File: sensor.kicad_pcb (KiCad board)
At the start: 2 copper layers, 42.2 x 40.8 mm, 14 parts, among them J1 Conn_01x06_Female, U2 TLV70019_SOT23-5, U3 TXB0106PWR, U4 PMW3360DM-T2QU

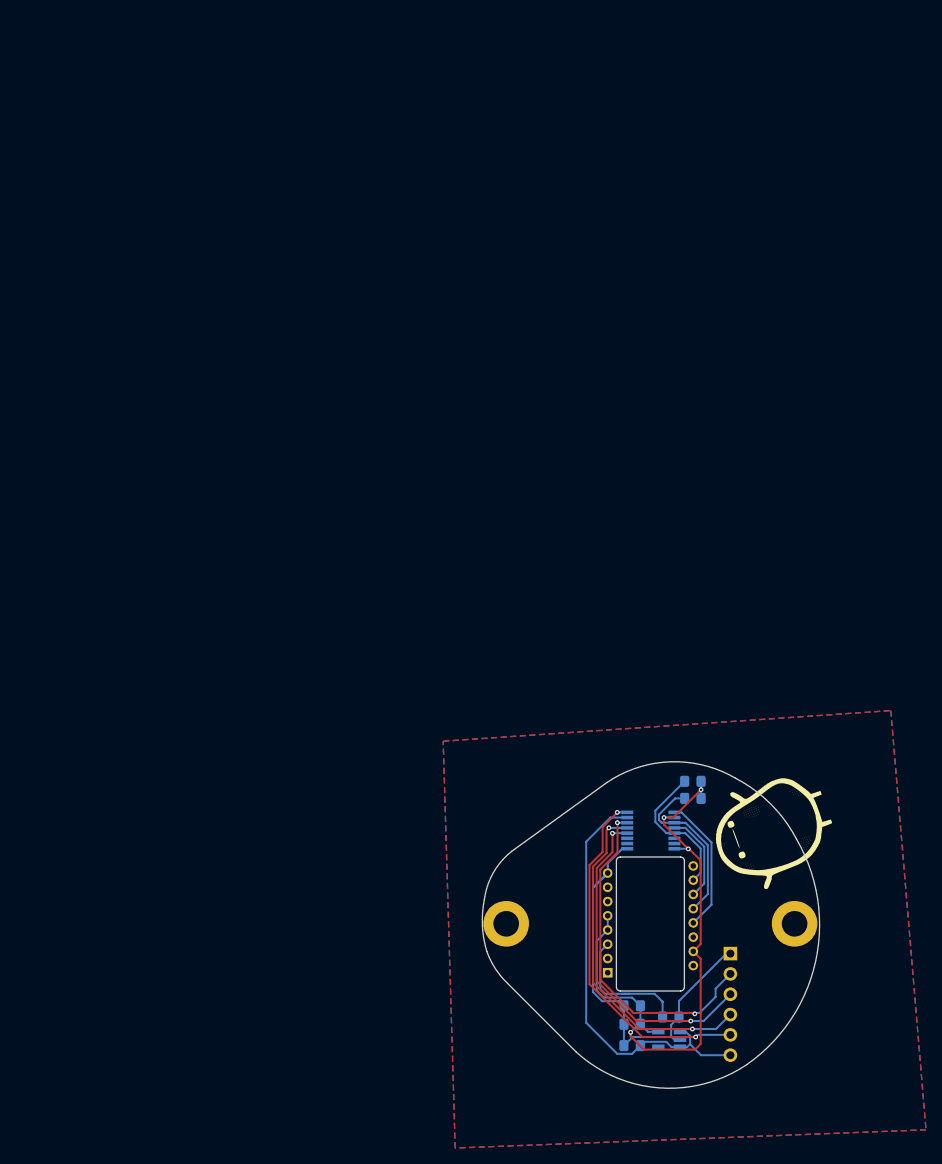
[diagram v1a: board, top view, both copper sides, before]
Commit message: restart project
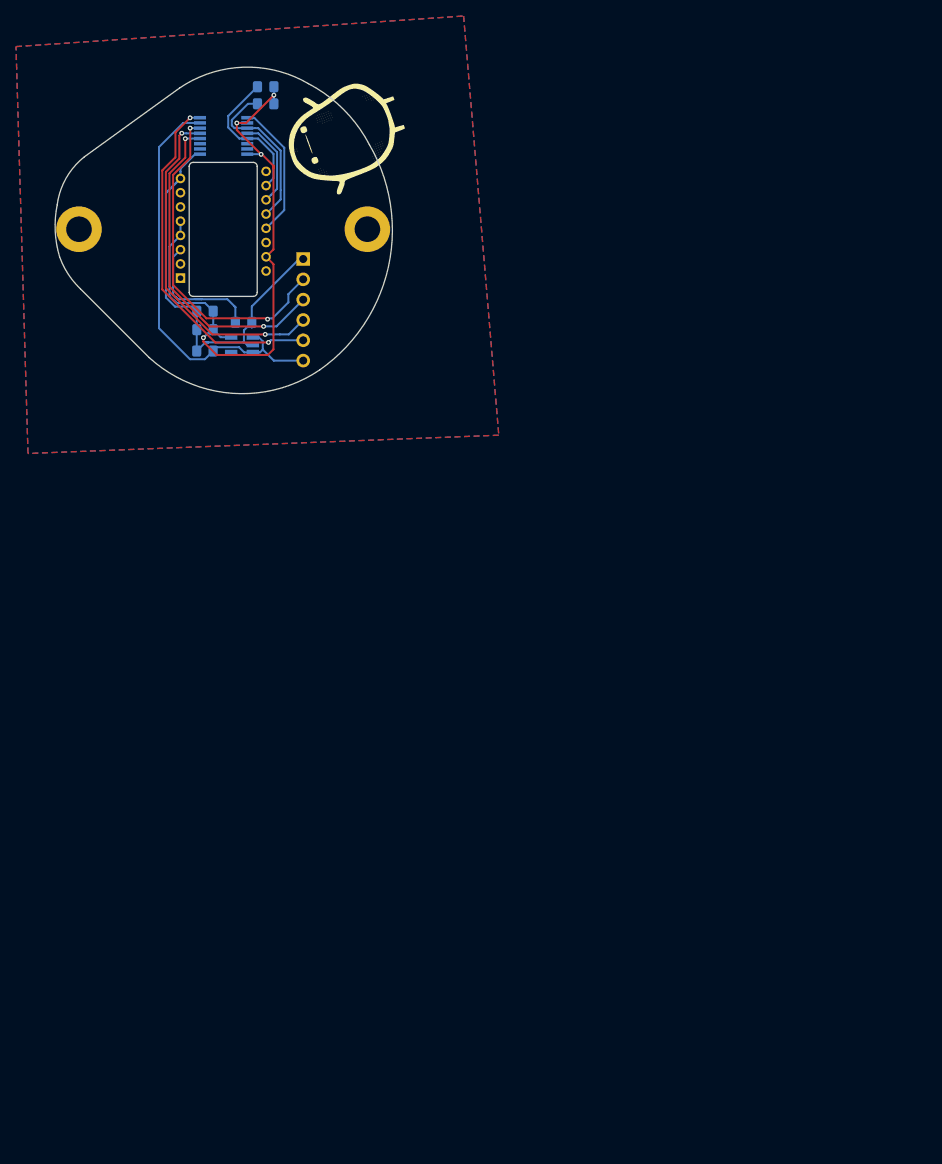
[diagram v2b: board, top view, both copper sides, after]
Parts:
- moved C2 101.9 mm to (25.9, 34.1)
- moved G*** 101.9 mm to (43.1, 13.1)
- moved J1 101.9 mm to (38.1, 27.6)
- moved REF** 101.9 mm to (10.1, 23.8)
- moved REF** 101.9 mm to (46.2, 23.8)
- moved U3 101.9 mm to (28.2, 12.2)
- moved C1 101.9 mm to (25.9, 39.1)
- moved C4 101.9 mm to (30.7, 35.5)
- moved R1 101.9 mm to (33.5, 8.15)
- moved R2 101.9 mm to (33.5, 6.01)
- moved R3 101.9 mm to (25.9, 36.4)
- moved U2 101.9 mm to (30.5, 38.3)
- moved U4 101.9 mm to (23.9, 31.5)
